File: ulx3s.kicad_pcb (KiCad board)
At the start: 4 copper layers, 139.5 x 70 mm, 274 parts, among them IC101 TPD4E001DRLR, IC102 74AUP1G74DC.125, IC103 CD74HC4050PWR, IC104 STM32F769IIT6, IC105 LD1117ADT33TR, IC106 N.C., IC107 IS42S16400J, IC108 AT24C256C-SSHL-B, IC109 TPS2051BDBVR, IC110 TPS61169DCKR, IC111 TPD4E001DRLR, IC112 TSC2007IPW, IC113 N.C., IC114 DP83848CVV_NOPB, J101 503398-1892, J102 67803-8020, J4 CONN_02X03, Q101 N.C., Q102 2N7002, SW101 TL1100CF160Q, SW102 PEC16-2215F-S0024, U1 LFE5U-85F-6BG381C, U10 IS25LP128F-JBLE, U3 TLV62569DBV, U4 TLV62569DBV, U5 TLV62569DBV, X101 DS1024-2*20R0, X102 DS1013-16SSIB1, X103 691322110005, X104 N.C., X105 LMJTAB881243M-L, Y1 FNETHE025, Y101 25MHz, Y102 XTAL016178-85SMX

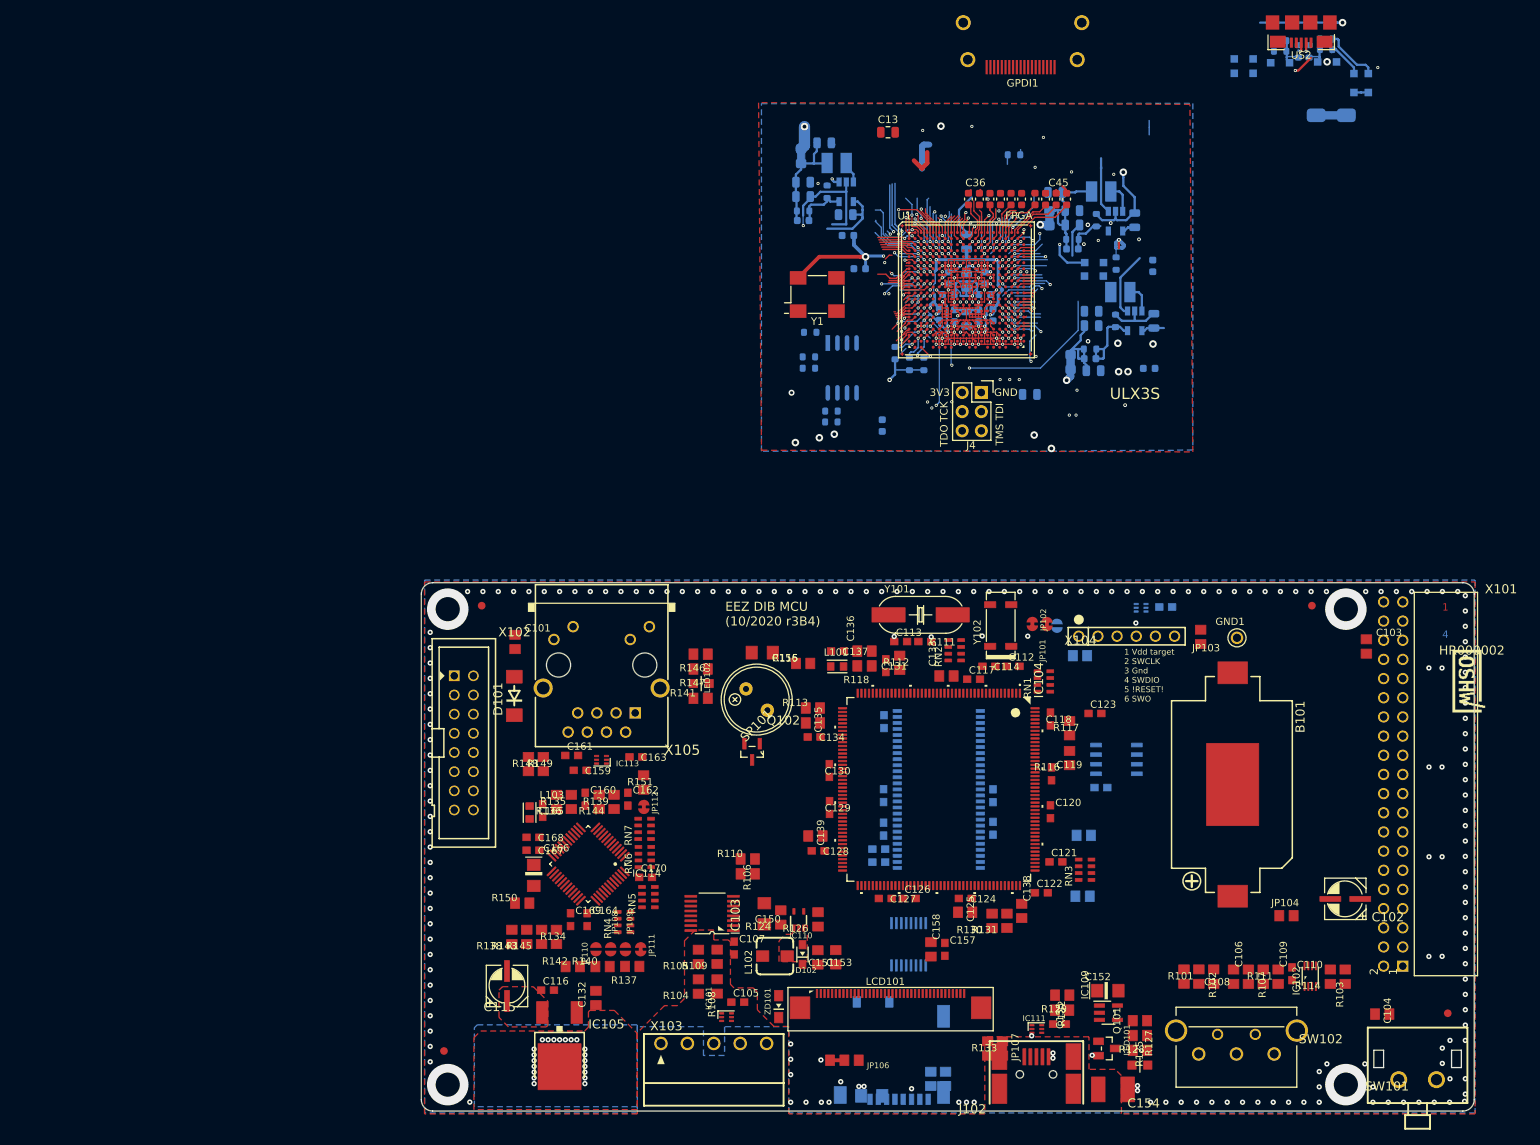
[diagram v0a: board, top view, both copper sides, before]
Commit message: Combined
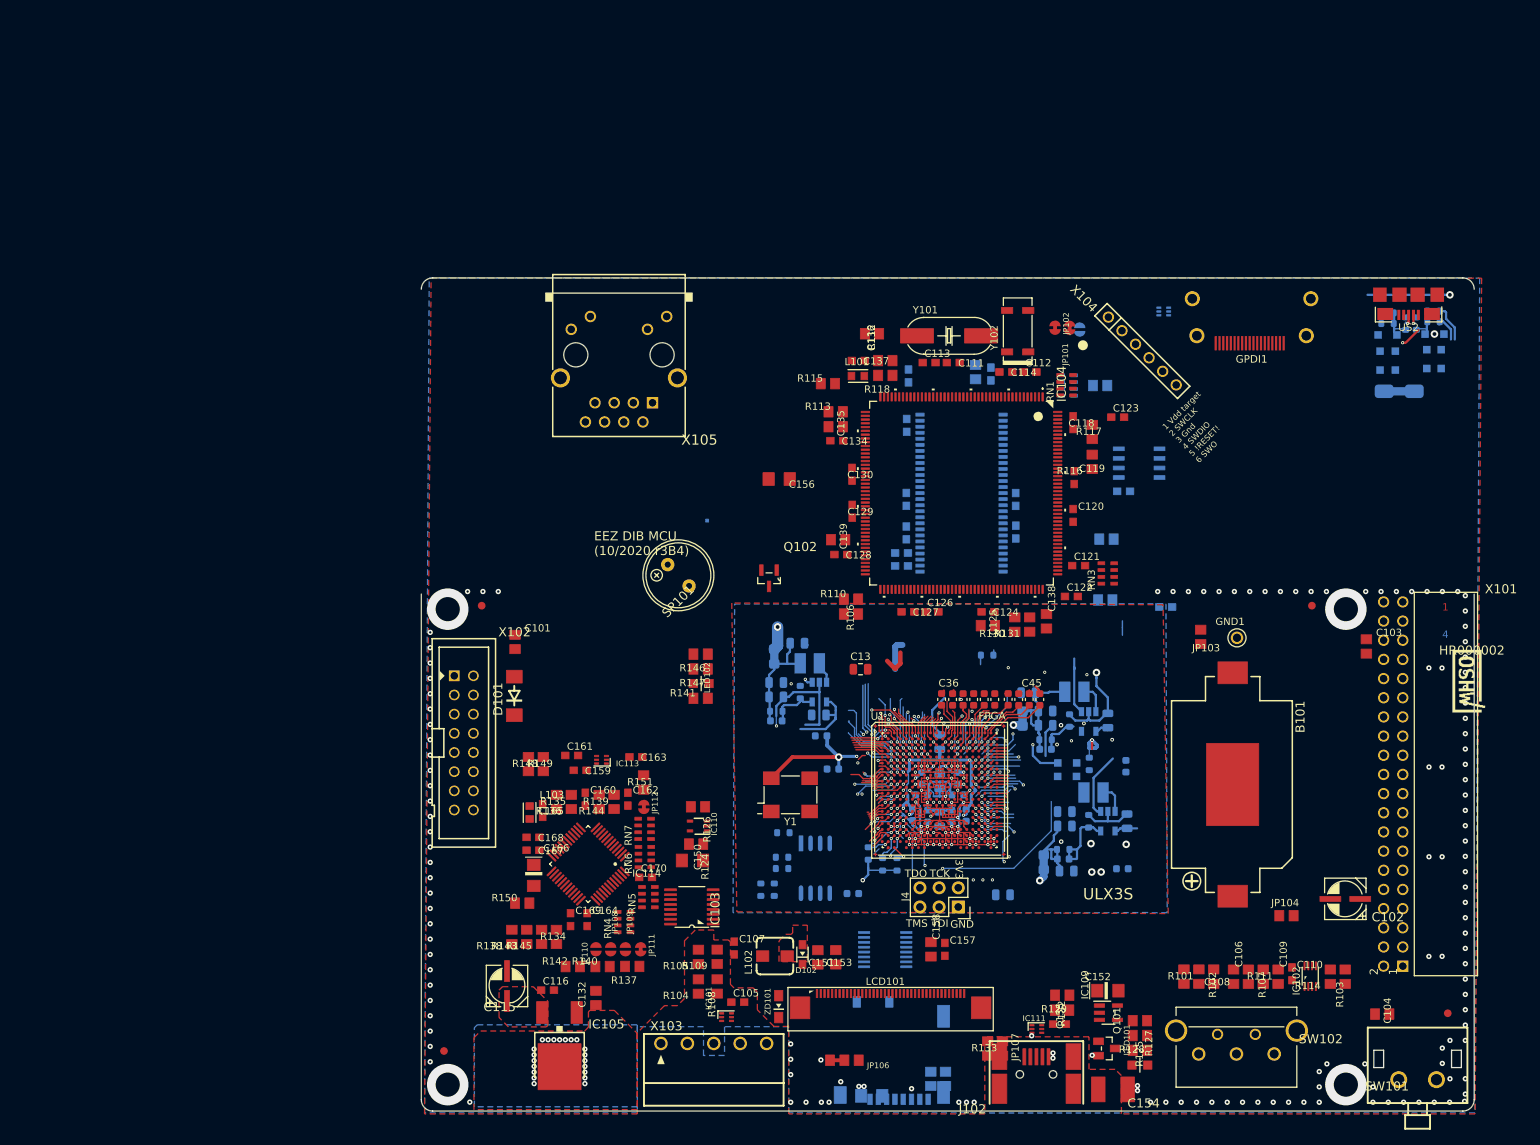
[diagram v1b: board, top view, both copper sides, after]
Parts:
- C117, C131, C133, RN2: moved to B.Cu
- moved C13 71.2 mm to (144.3, 74.0)
- moved J4 68.2 mm to (157.3, 105.5), turned to 180 degrees
- moved C1 66.4 mm to (138.8, 80.1)
- moved C2 66.4 mm to (171.2, 99.2)
- moved C3 66.4 mm to (171.4, 92.9)
- moved C30 66.4 mm to (151.2, 93.3)
- moved C4 66.4 mm to (171.4, 94.8)
- moved C42 66.4 mm to (155.1, 78.0)
- moved C46 66.4 mm to (163.2, 103.9)
- moved C48 66.4 mm to (139.1, 82.9)
- moved C53 66.4 mm to (140.7, 87.2)
- moved D28 66.4 mm to (171.7, 86.4)
- moved L3 66.4 mm to (172.7, 77.0)
- moved R11 66.4 mm to (133.9, 100.4)
- moved R27 66.4 mm to (145.4, 98.4)
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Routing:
- net +5V: track 258.7 -> 159.5 mm
- net +12V: track 136.6 -> 37.4 mm
- net JTAG_TDI: track 12.6 -> 7.73 mm, vias 3 -> 2
- net JTAG_TMS: track 11.0 -> 6.28 mm, vias 2 -> 1
- net JTAG_TCK: track 11.8 -> 7.39 mm, vias 2 -> 1
- net /gpio/OUT5V: track 4.31 -> 0.00 mm, vias 1 -> 0
- net JTAG_TDO: track 9.95 -> 5.69 mm, vias 3 -> 2
- net /gpio/IN5V: track 18.9 -> 15.3 mm
- net Net-(D26-Pad1): track 7.59 -> 4.94 mm
- net USB_FPGA_PULL_D-: track 2.47 -> 0.57 mm
- net Net-(D25-Pad2): track 4.76 -> 3.36 mm
- net 2V5_3V3: track 28.2 -> 28.0 mm, vias 4 -> 2
- net SPI2_CSB: track 0.05 -> 0.00 mm, vias 1 -> 0
- net GND: vias 270 -> 212
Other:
- board size 139.5 x 70 mm -> 139.5 x 110.4 mm

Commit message: Board update
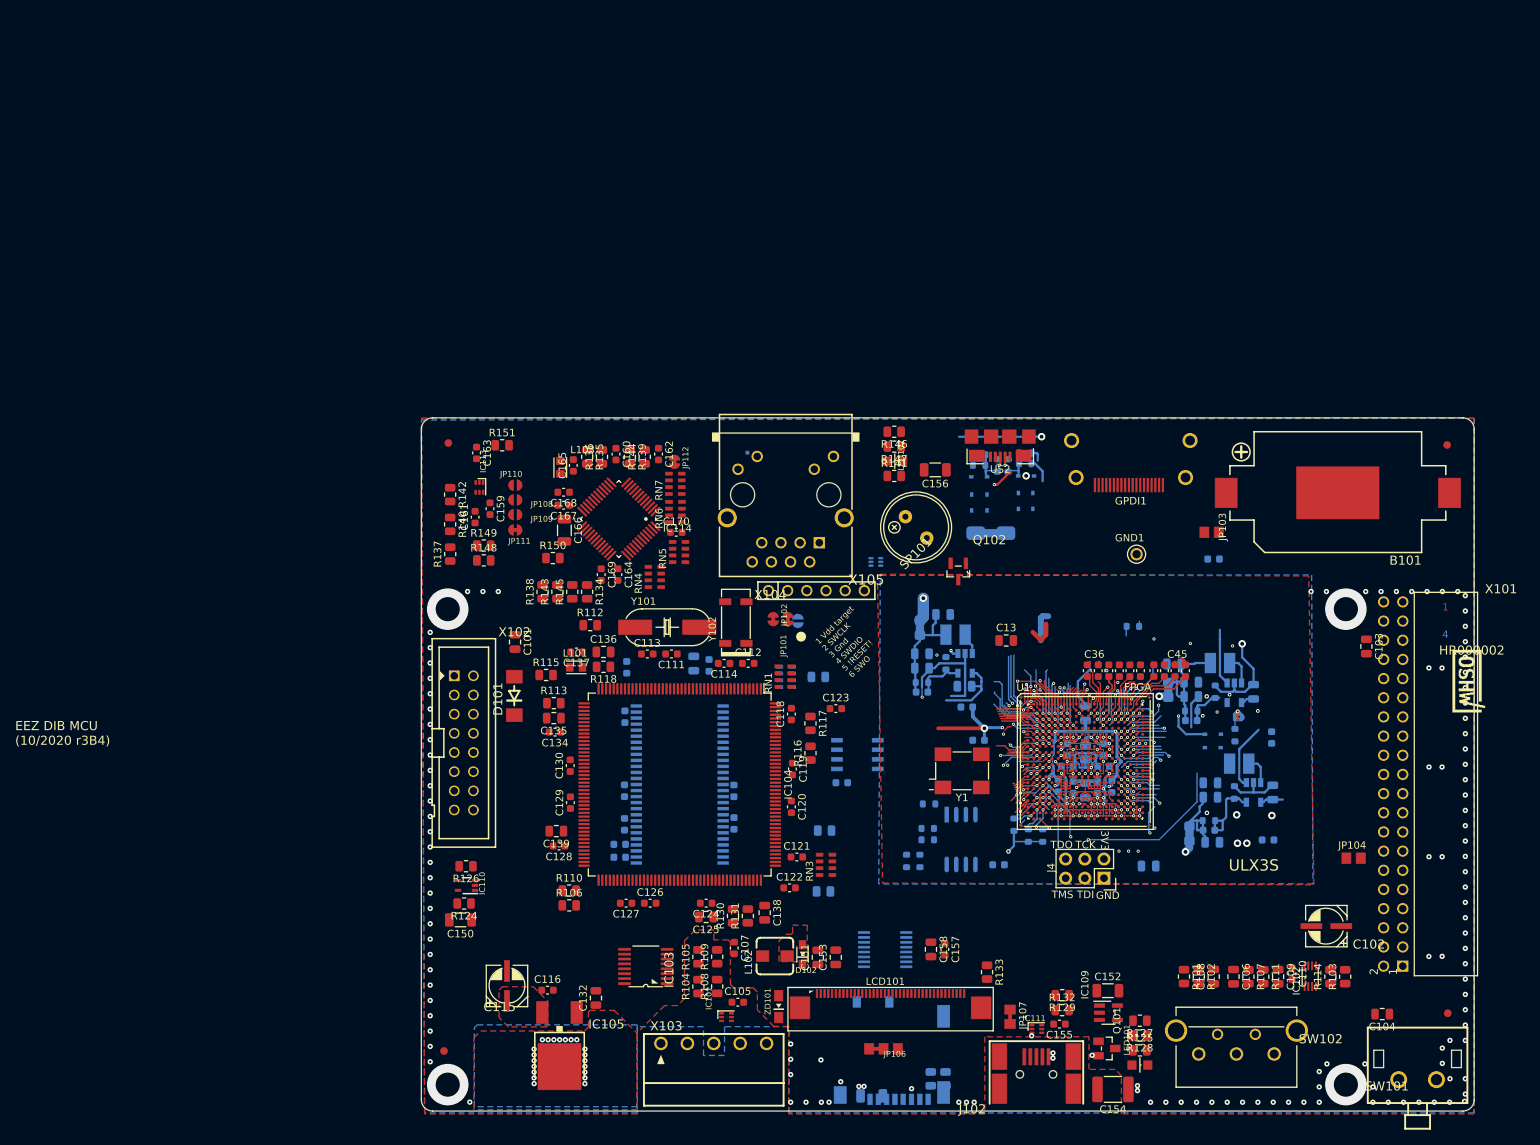
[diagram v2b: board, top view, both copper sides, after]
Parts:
- C101, C103, C104, C106, C108, C109, C125, C132, C133, C135, C136, C138, C139, C151, C153, C158: footprint EEZ DIB MCU r3B4:C0805 -> Capacitor_SMD:C_0805_2012Metric
- C105, C107, C110, C111, C112, C113, C114, C116, C117, C118, C119, C120, C121, C122, C123, C124, C126, C127, C128, C129, C130, C131, C134, C137, C140, C142, C143, C144, C145, C146, C147, C148, C149, C155, C157, C159, C160, C161, C162, C163, C164, C165, C167, C168, C169, C170: footprint EEZ DIB MCU r3B4:C0603 -> Capacitor_SMD:C_0603_1608Metric
- C141, C150, C156: footprint EEZ DIB MCU r3B4:C1206 -> Capacitor_SMD:C_1206_3216Metric
- C152, C166: footprint EEZ DIB MCU r3B4:EC1206 -> Capacitor_SMD:C_1206_3216Metric
- C154: footprint EEZ DIB MCU r3B4:C1812 -> Capacitor_SMD:C_1812_4532Metric
- D20, D21, D23, D24, D25, D26, D28, D29: footprint Diode_SMD:D_SOD-323_HandSoldering -> Diode_SMD:D_SOD-323
- IC104: footprint EEZ DIB MCU r3B4:LQFP-176_24X24MM -> Package_QFP:LQFP-176_24x24mm_P0.5mm
- IC107: footprint EEZ DIB MCU r3B4:TSOPII-54 -> Package_SO:TSOP-II-54_22.2x10.16mm_P0.8mm
- R101, R102, R103, R104, R105, R106, R107, R108, R109, R110, R111, R112, R113, R114, R115, R116, R117, R118, R119, R120, R121, R122, R123, R124, R125, R126, R127, R128, R129, R130, R131, R132, R133, R134, R135, R136, R137, R138, R139, R140, R141, R142, R143, R144, R145, R146, R147, R148, R149, R150, R151: footprint EEZ DIB MCU r3B4:R0805 -> Resistor_SMD:R_0805_2012Metric
- moved R142 64.6 mm to (90.0, 50.9), turned to 270 degrees
- moved JP110 62.4 mm to (98.6, 49.6), turned to 0 degrees
- moved R140 62.0 mm to (90.0, 54.8), turned to 270 degrees
- moved JP108 60.9 mm to (98.6, 51.6), turned to 180 degrees
- moved R137 59.7 mm to (90.0, 58.8), turned to 90 degrees
- moved JP109 59.4 mm to (98.6, 53.6), turned to 180 degrees
- moved JP111 58.0 mm to (98.6, 55.6), turned to 180 degrees
- moved D21 57.3 mm to (166.3, 48.4)
- moved D23 57.3 mm to (161.1, 51.9)
- moved D25 57.3 mm to (165.3, 51.7)
- moved D26 57.3 mm to (167.2, 51.7)
- moved D9 57.3 mm to (161.6, 56.0)
- moved R52 57.3 mm to (163.9, 47.0)
- moved R53 57.3 mm to (162.5, 47.0)
- moved R54 57.3 mm to (166.2, 45.4)
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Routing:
- net +12V: track 37.4 -> 14.0 mm
- net +5V: track 159.5 -> 139.0 mm
- net +2V5: track 92.7 -> 103.0 mm
- net +3V3: track 88.4 -> 84.5 mm
- net Net-(D26-Pad1): track 4.94 -> 1.72 mm
- net USB_FPGA_PULL_D+: track 7.45 -> 5.54 mm
- net GND: vias 212 -> 202
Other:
- board size 139.5 x 110.4 mm -> 139.5 x 91.8 mm
